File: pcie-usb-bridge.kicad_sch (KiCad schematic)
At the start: 50 parts, among them IC1 UPD720201K8-711-BAC-A, U2 SST25VF512A, Y1 NX3225SA-24M

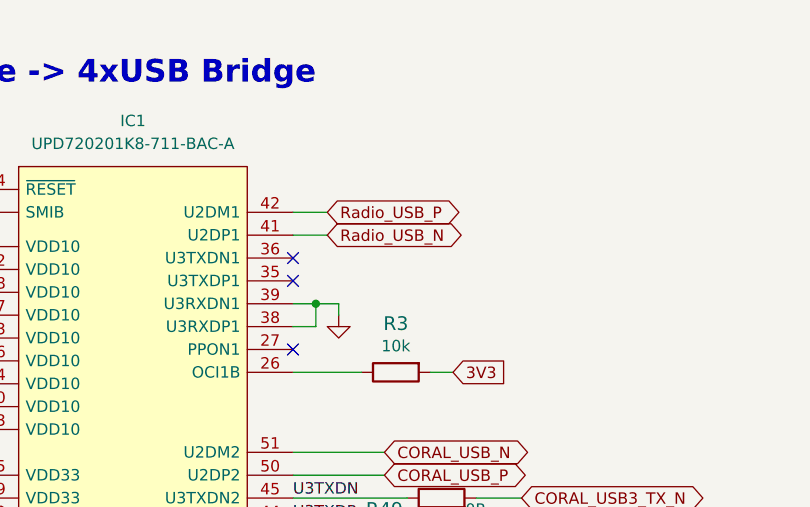
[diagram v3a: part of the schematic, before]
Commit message: Applied fixes to issues that came up in review
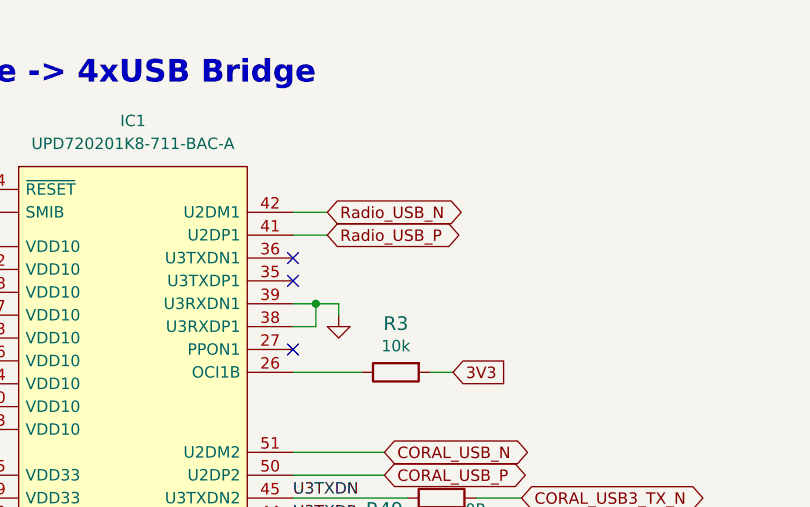
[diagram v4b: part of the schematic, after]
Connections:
- net Radio_USB_N: now also IC1.42 (U2DM1); no longer IC1.41 (U2DP1)
- net Radio_USB_P: now also IC1.41 (U2DP1); no longer IC1.42 (U2DM1)
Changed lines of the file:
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@@
     )
   )
-  (global_label "Radio_USB_P" (shape bidirectional) (at 114.3 34.29 0) (fields_autoplaced)
+  (global_label "Radio_USB_P" (shape bidirectional) (at 114.3 36.83 0) (fields_autoplaced)
     (effects (font (size 1.27 1.27)) (justify left))
-    (property "Intersheet References" "${INTERSHEET_REFS}" (id 0) (at 128.9613 34.2106 0)
+    (property "Intersheet References" "${INTERSHEET_REFS}" (id 0) (at 128.9613 36.7506 0)
       (effects (font (size 1.27 1.27)) (justify left) hide)
     )
@@
     )
   )
-  (global_label "Radio_USB_N" (shape bidirectional) (at 114.3 36.83 0) (fields_autoplaced)
+  (global_label "Radio_USB_N" (shape bidirectional) (at 114.3 34.29 0) (fields_autoplaced)
     (effects (font (size 1.27 1.27)) (justify left))
-    (property "Intersheet References" "${INTERSHEET_REFS}" (id 0) (at 129.0218 36.7506 0)
+    (property "Intersheet References" "${INTERSHEET_REFS}" (id 0) (at 129.0218 34.2106 0)
       (effects (font (size 1.27 1.27)) (justify left) hide)
     )
